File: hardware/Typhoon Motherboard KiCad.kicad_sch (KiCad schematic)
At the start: 45 parts, among them J1 Conn_01x04_Pin, J2 Conn_02x03_Odd_Even, P1 USB_C_Plug_USB2.0, U1 ESP32-S3-WROOM-1, U2 TPS54360DDA, U3 TJA1051T-3, U7 MCP1825S

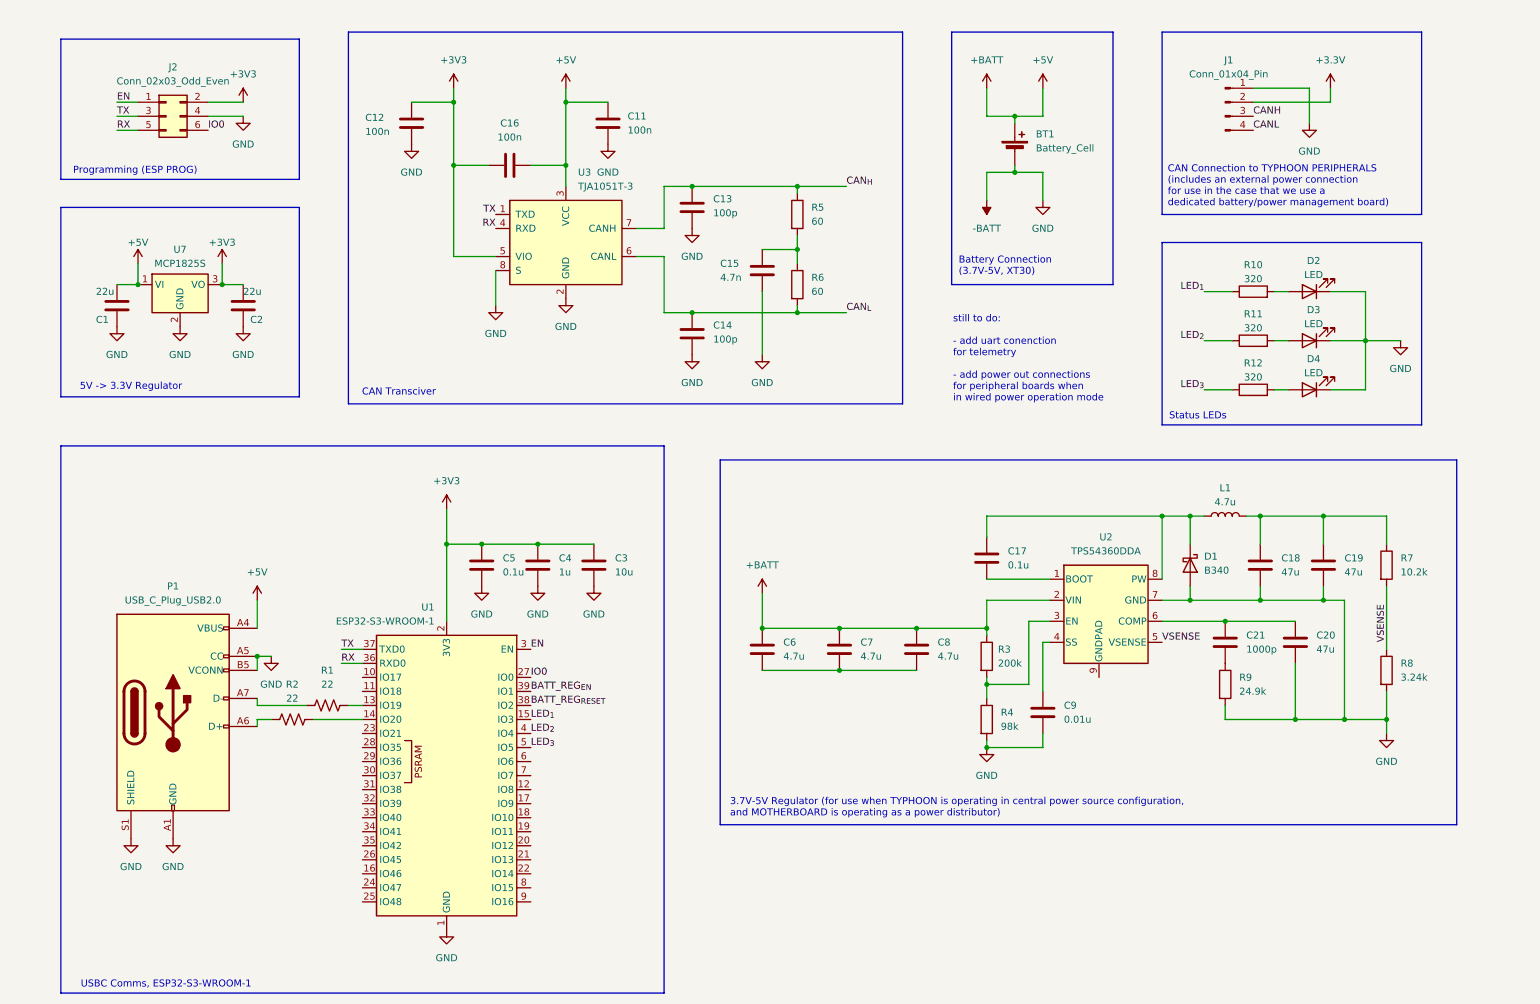
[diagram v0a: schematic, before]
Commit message: Rev 2 upload
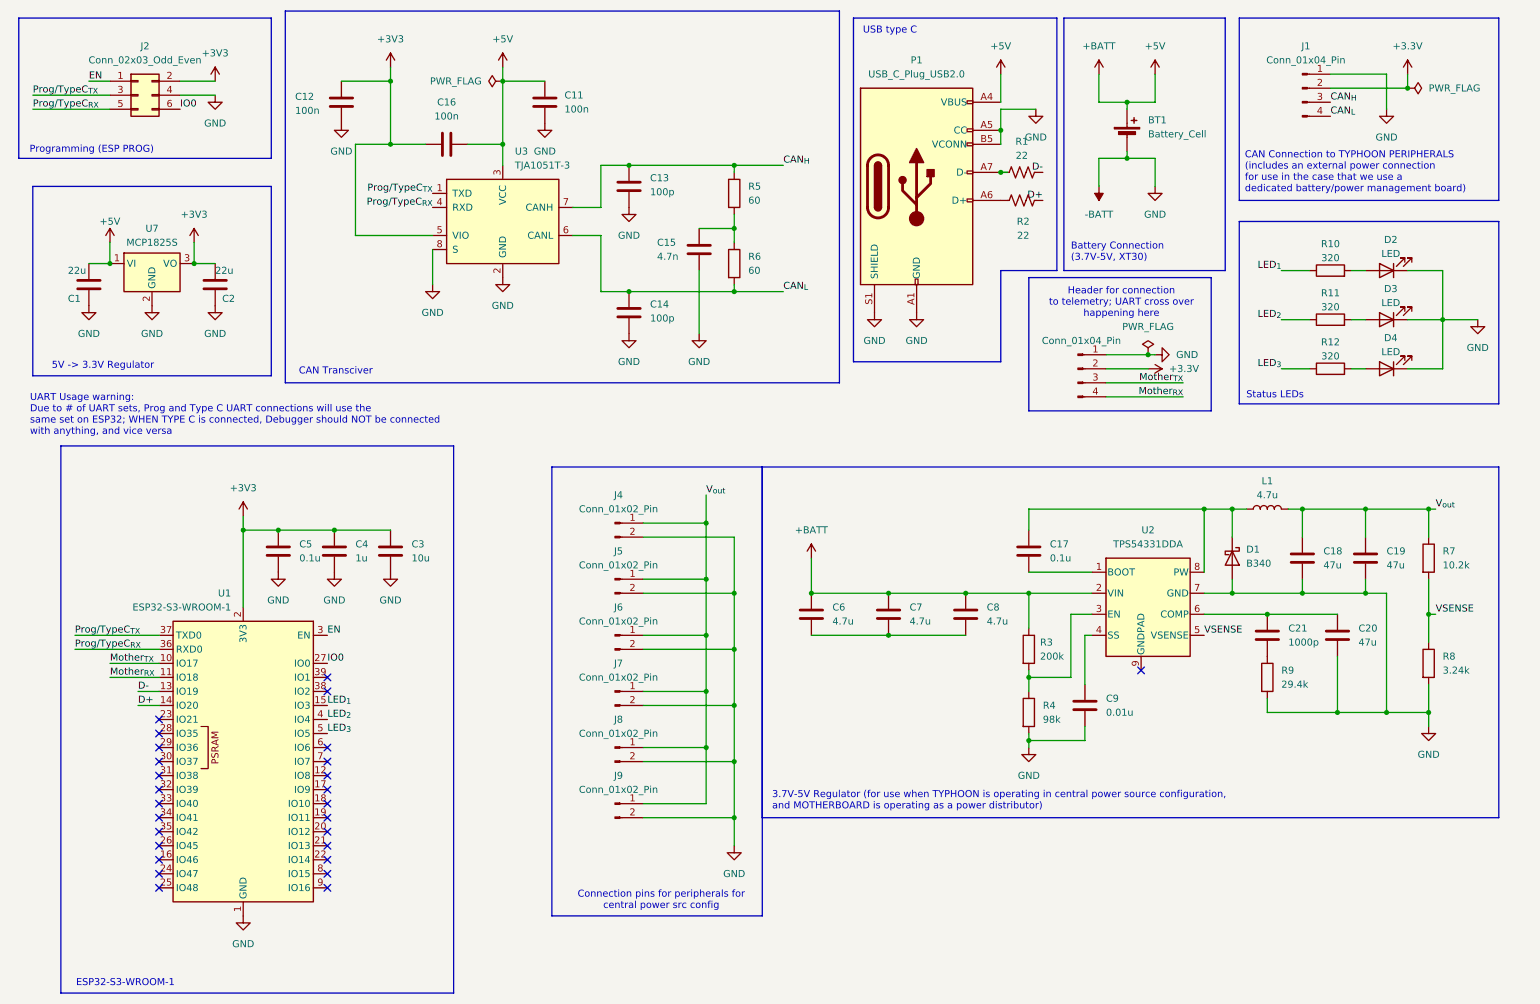
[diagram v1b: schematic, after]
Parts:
- added J3: Conn_01x04_Pin, Connector_PinHeader_1.27mm:PinHeader_1x04_P1.27mm_Vertical, symbol Connector:Conn_01x04_Pin
- added J4, J5, J6, J7, J8, J9: Conn_01x02_Pin, Connector_PinHeader_2.00mm:PinHeader_1x02_P2.00mm_Vertical_SMD_Pin1Right, symbol Connector:Conn_01x02_Pin
- C11, C12, C13, C14, C15, C16, C17, C18, C19, C20, C21, C3, C4, C5, C6, C7, C8, C9: footprint (none) -> Capacitor_SMD:C_0603_1608Metric
- D2, D3, D4: footprint (none) -> LED_SMD:LED_0805_2012Metric
- L1: footprint (none) -> Inductor_SMD:L_Taiyo-Yuden_NR-60xx
- R1, R10, R11, R12, R2, R3, R4, R5, R6, R7, R8: footprint (none) -> Resistor_SMD:R_0603_1608Metric
- R9: value 24.9k -> 29.4k; footprint (none) -> Resistor_SMD:R_0603_1608Metric
- U2: value TPS54360DDA -> TPS54331DDA
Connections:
- net CANH is gone; now on net CAN_{H}: J1.3 (Pin_3)
- net CANL is gone; now on net CAN_{L}: J1.4 (Pin_4)
- net +3.3V: now also J3.2 (Pin_2)
- net -BATT: now also J3.1 (Pin_1), J4.2 (Pin_2), J5.2 (Pin_2), J6.2 (Pin_2), J7.2 (Pin_2), J8.2 (Pin_2), J9.2 (Pin_2)
- net D-: now reaches R1.2, U1.13 (IO19)
- net D+: now reaches R2.2, U1.14 (IO20)
- net Mother_{TX}: now reaches U1.10 (IO17)
- net Mother_{TX}: now also J3.3 (Pin_3)
- net Mother_{RX}: now reaches U1.11 (IO18)
- net Mother_{RX}: now also J3.4 (Pin_4)
- net V_{out}: now reaches C18.1, C19.1, L1.2, R7.1
- net V_{out}: now also J4.1 (Pin_1), J5.1 (Pin_1), J6.1 (Pin_1), J7.1 (Pin_1), J8.1 (Pin_1), J9.1 (Pin_1)
- net BATT_REG_{EN}: no longer names the net of U1.39 (IO1)
- net BATT_REG_{RESET}: no longer names the net of U1.38 (IO2)
- net RX renamed Prog/TypeC_{RX}
- net TX renamed Prog/TypeC_{TX}
- no-connect marks 0 -> 27
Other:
- note added: "Connection pins for peripherals for central power src config"
- note added: "ESP32-S3-WROOM-1"
- note added: "Header for connection to telemetry; UART cross over happening here"
- note added: "UART Usage warning: Due to # of UART sets, Prog and Type C UART connections will use the same set on ESP32; WHEN TYPE C is connected, Debugger should NOT be connected with anything, and vice versa"
- note added: "USB type C"
- note removed: "USBC Comms, ESP32-S3-WROOM-1"
- note removed: "still to do: - add uart conenction for telemetry - add power out connections for peripheral boards when in wired power operation mode"
- moved on the sheet: BT1, C1, C11, C12, C13, C14, C15, C16, C17, C18, C19, C2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
